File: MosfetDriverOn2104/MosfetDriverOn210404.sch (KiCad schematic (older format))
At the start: 88 parts, among them J1 I2C HDR, J10 ENCODER HDR, J11 CROSS CONN, J12 motor, J2 AVR-ISP-6, J3 I2C HDR, J4 Screw_Terminal_01x02, J5 I2C HDR, J6 UART HDR, J7 5V HDR, J8 GND HDR, J9 servo hdr, Q1 IRF540N, Q2 IRF540N, Q3 IRF540N, Q4 IRF540N, SW1 SW_Push, SW2 SW_DIP_x04, SW3 SW_Push, SW4 SW_Push, U1 LM2576HVS-ADJ, U2 L7805, U3 IR2104, U4 LM358, U5 IR2104, U6 ATmega328P-AU-MCU_Microchip_A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

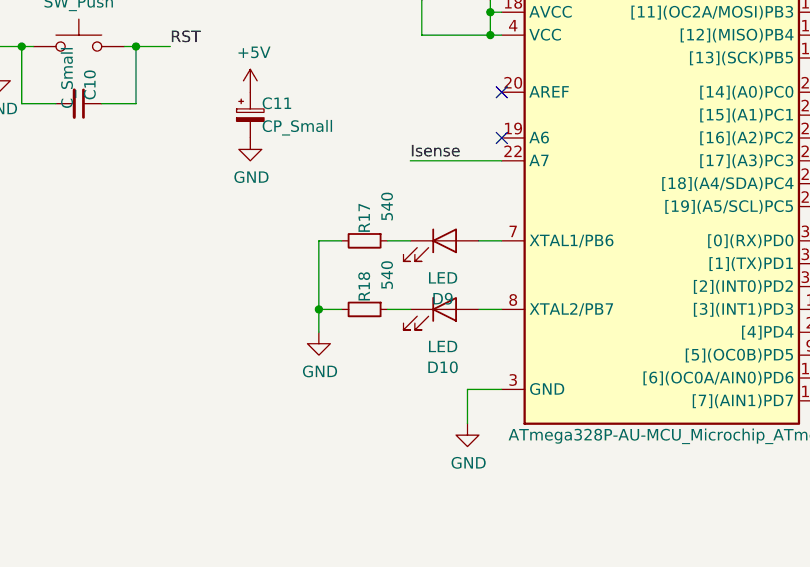
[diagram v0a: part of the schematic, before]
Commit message: yet to arrange!
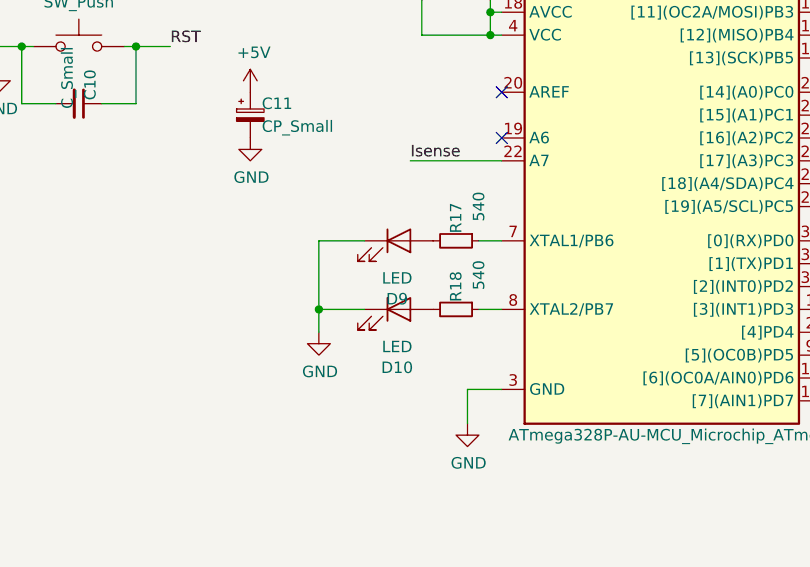
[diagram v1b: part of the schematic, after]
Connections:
- net GND: now also D10.1 (K), D9.1 (K); no longer R17.2, R18.2
- net at U6.7 (XTAL1/PB6): now also R17.1; no longer D9.2 (A)
- net at U6.8 (XTAL2/PB7): now also R18.1; no longer D10.2 (A)
- new net: D9.2 (A), R17.2
- new net: D10.2 (A), R18.2
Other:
- moved on the sheet: D10, D9, R17, R18
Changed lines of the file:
@@
 L Device:LED D?
 U 1 1 5BD9759E
-P 16800 850
+P 16600 850
 AR Path="/5BCF2976/5BD9759E" Ref="D?"  Part="1"
 AR Path="/5BD9759E" Ref="D9"  Part="1"
-F 0 "D9" H 16792 595 50  0000 C CNN
-F 1 "LED" H 16792 686 50  0000 C CNN
-F 2 "LED_SMD:LED_0805_2012Metric" H 16800 850 50  0001 C CNN
-F 3 "~" H 16800 850 50  0001 C CNN
-	1    16800 850
+F 0 "D9" H 16592 595 50  0000 C CNN
+F 1 "LED" H 16592 686 50  0000 C CNN
+F 2 "LED_SMD:LED_0805_2012Metric" H 16600 850 50  0001 C CNN
+F 3 "~" H 16600 850 50  0001 C CNN
+	1    16600 850
 	1    0    0    -1
 $EndComp
@@
 L Device:R_Small R?
 U 1 1 5BD975A5
-P 16450 850
+P 16850 850
 AR Path="/5BCF2976/5BD975A5" Ref="R?"  Part="1"
 AR Path="/5BD975A5" Ref="R17"  Part="1"
-F 0 "R17" H 16350 850 50  0000 C CNN
-F 1 "540" H 16300 950 50  0000 C CNN
-F 2 "Resistor_SMD:R_0805_2012Metric" H 16450 850 50  0001 C CNN
-F 3 "~" H 16450 850 50  0001 C CNN
-	1    16450 850
+F 0 "R17" H 16750 850 50  0000 C CNN
+F 1 "540" H 16700 950 50  0000 C CNN
+F 2 "Resistor_SMD:R_0805_2012Metric" H 16850 850 50  0001 C CNN
+F 3 "~" H 16850 850 50  0001 C CNN
+	1    16850 850
 	0    1    1    0
 $EndComp
@@
 L Device:LED D?
 U 1 1 5BD975B2
-P 16800 1150
+P 16600 1150
 AR Path="/5BCF2976/5BD975B2" Ref="D?"  Part="1"
 AR Path="/5BD975B2" Ref="D10"  Part="1"
-F 0 "D10" H 16792 895 50  0000 C CNN
-F 1 "LED" H 16792 986 50  0000 C CNN
-F 2 "LED_SMD:LED_0805_2012Metric" H 16800 1150 50  0001 C CNN
-F 3 "~" H 16800 1150 50  0001 C CNN
-	1    16800 1150
+F 0 "D10" H 16592 895 50  0000 C CNN
+F 1 "LED" H 16592 986 50  0000 C CNN
+F 2 "LED_SMD:LED_0805_2012Metric" H 16600 1150 50  0001 C CNN
+F 3 "~" H 16600 1150 50  0001 C CNN
+	1    16600 1150
 	1    0    0    -1
 $EndComp
@@
 L Device:R_Small R?
 U 1 1 5BD975B9
-P 16450 1150
+P 16850 1150
 AR Path="/5BCF2976/5BD975B9" Ref="R?"  Part="1"
 AR Path="/5BD975B9" Ref="R18"  Part="1"
-F 0 "R18" H 16350 1150 50  0000 C CNN
-F 1 "540" H 16300 1250 50  0000 C CNN
-F 2 "Resistor_SMD:R_0805_2012Metric" H 16450 1150 50  0001 C CNN
-F 3 "~" H 16450 1150 50  0001 C CNN
-	1    16450 1150
+F 0 "R18" H 16750 1150 50  0000 C CNN
+F 1 "540" H 16700 1250 50  0000 C CNN
+F 2 "Resistor_SMD:R_0805_2012Metric" H 16850 1150 50  0001 C CNN
+F 3 "~" H 16850 1150 50  0001 C CNN
+	1    16850 1150
 	0    1    1    0
 $EndComp
-Wire Wire Line
-	16650 1150 16550 1150
-Wire Wire Line
-	16650 850  16550 850
 Wire Wire Line
 	17050 850  16950 850
@@
 $EndComp
 Wire Wire Line
-	16350 850  16250 850
-Wire Wire Line
 	16250 850  16250 1150
-Wire Wire Line
-	16350 1150 16250 1150
 Connection ~ 16250 1150
 Wire Wire Line
@@
 	1    0    0    -1
 $EndComp
+Wire Wire Line
+	16250 850  16450 850
+Wire Wire Line
+	16250 1150 16450 1150
 $EndSCHEMATC

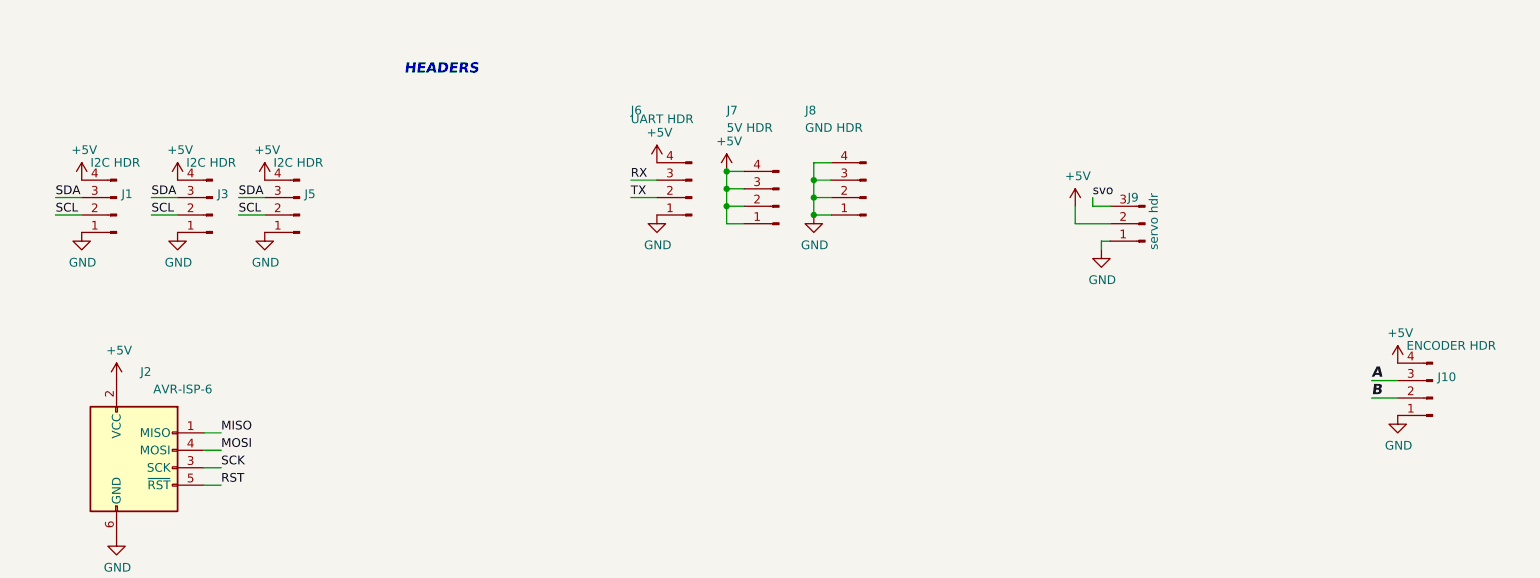
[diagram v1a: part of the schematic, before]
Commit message: necktie pattern
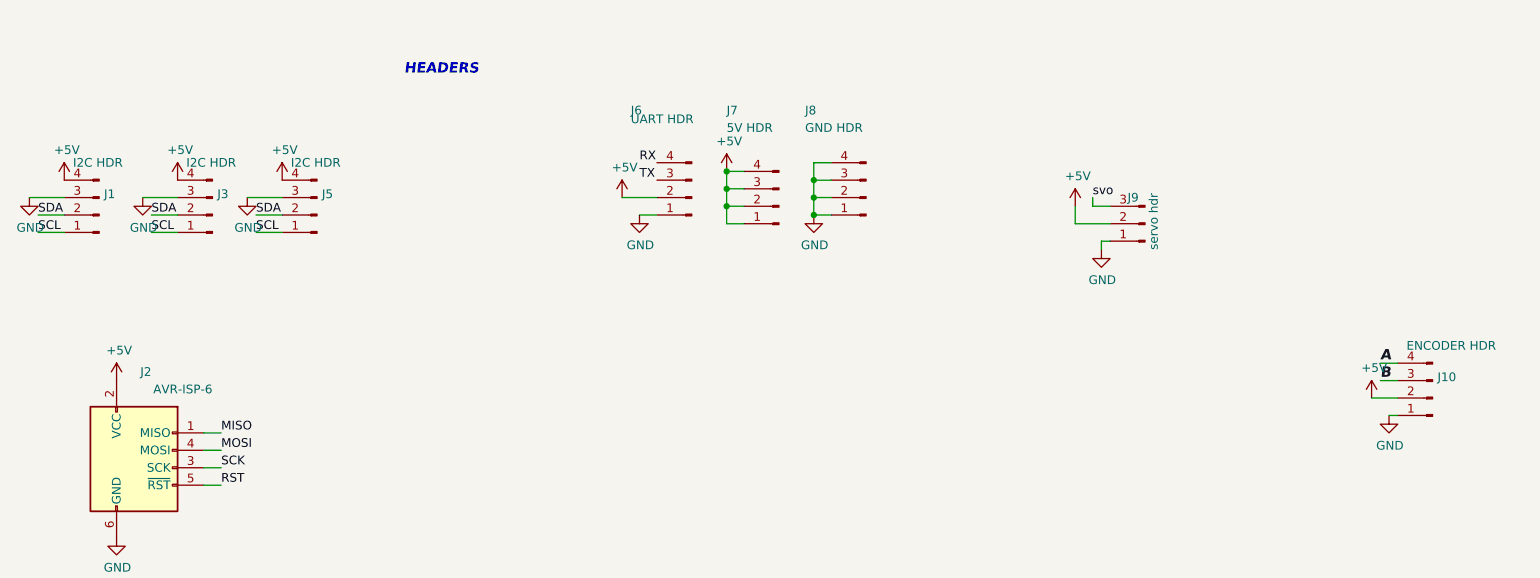
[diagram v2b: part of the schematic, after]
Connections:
- net +5V: now also J10.2 (Pin_2), J6.2 (Pin_2); no longer J10.4 (Pin_4), J6.4 (Pin_4)
- net A: now also J10.4 (Pin_4); no longer J10.3 (Pin_3)
- net B: now also J10.3 (Pin_3); no longer J10.2 (Pin_2)
- net GND: now also J1.3 (Pin_3), J3.3 (Pin_3), J5.3 (Pin_3); no longer J1.1 (Pin_1), J3.1 (Pin_1), J5.1 (Pin_1)
- net RX: no longer J6.3 (Pin_3)
- net SCL: now also J1.1 (Pin_1), J3.1 (Pin_1), J5.1 (Pin_1); no longer J1.2 (Pin_2), J3.2 (Pin_2), J5.2 (Pin_2)
- net SDA: now also J1.2 (Pin_2), J3.2 (Pin_2), J5.2 (Pin_2); no longer J1.3 (Pin_3), J3.3 (Pin_3), J5.3 (Pin_3)
- net TX: no longer J6.2 (Pin_2)
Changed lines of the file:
@@
 L power:+5V #PWR0118
 U 1 1 5BD95BFB
-P -5900 -550
+P -6100 -350
 AR Path="/5BD95BFB" Ref="#PWR0118"  Part="1"
 AR Path="/5BD0E604/5BD95BFB" Ref="#PWR?"  Part="1"
-F 0 "#PWR0118" H -5900 -700 50  0001 C CNN
-F 1 "+5V" H -5885 -377 50  0000 C CNN
-F 2 "" H -5900 -550 50  0001 C CNN
-F 3 "" H -5900 -550 50  0001 C CNN
-	1    -5900 -550
+F 0 "#PWR0118" H -6100 -500 50  0001 C CNN
+F 1 "+5V" H -6085 -177 50  0000 C CNN
+F 2 "" H -6100 -350 50  0001 C CNN
+F 3 "" H -6100 -350 50  0001 C CNN
+	1    -6100 -350
 	1    0    0    -1
 $EndComp
@@
 L power:GND #PWR0119
 U 1 1 5BD95C01
-P -5900 -250
+P -6000 -250
 AR Path="/5BD95C01" Ref="#PWR0119"  Part="1"
 AR Path="/5BD0E604/5BD95C01" Ref="#PWR?"  Part="1"
-F 0 "#PWR0119" H -5900 -500 50  0001 C CNN
-F 1 "GND" H -5895 -423 50  0000 C CNN
-F 2 "" H -5900 -250 50  0001 C CNN
-F 3 "" H -5900 -250 50  0001 C CNN
-	1    -5900 -250
-	1    0    0    -1
-$EndComp
-Text Label -6050 -450 0    50   ~ 0
+F 0 "#PWR0119" H -6000 -500 50  0001 C CNN
+F 1 "GND" H -5995 -423 50  0000 C CNN
+F 2 "" H -6000 -250 50  0001 C CNN
+F 3 "" H -6000 -250 50  0001 C CNN
+	1    -6000 -250
+	1    0    0    -1
+$EndComp
+Text Label -6000 -550 0    50   ~ 0
 RX
-Text Label -6050 -350 0    50   ~ 0
+Text Label -6000 -450 0    50   ~ 0
 TX
-Wire Wire Line
-	-6050 -450 -5900 -450
-Wire Wire Line
-	-5900 -350 -6050 -350
-$Comp
-L Connector:Conn_01x04_Male J5
-U 1 1 5BD95C0B
-P -7950 -250
-AR Path="/5BD95C0B" Ref="J5"  Part="1"
-AR Path="/5BD0E604/5BD95C0B" Ref="J?"  Part="1"
-F 0 "J5" H -7978 -370 50  0000 R CNN
-F 1 "I2C HDR" H -7800 -550 50  0000 R CNN
-F 2 "Connector_PinHeader_2.54mm:PinHeader_1x04_P2.54mm_Vertical" H -7950 -250 50  0001 C CNN
-F 3 "~" H -7950 -250 50  0001 C CNN
-	1    -7950 -250
-	-1   0    0    1
-$EndComp
-$Comp
-L power:+5V #PWR0120
-U 1 1 5BD95C12
-P -8150 -450
-AR Path="/5BD95C12" Ref="#PWR0120"  Part="1"
-AR Path="/5BD0E604/5BD95C12" Ref="#PWR?"  Part="1"
-F 0 "#PWR0120" H -8150 -600 50  0001 C CNN
-F 1 "+5V" H -8135 -277 50  0000 C CNN
-F 2 "" H -8150 -450 50  0001 C CNN
-F 3 "" H -8150 -450 50  0001 C CNN
-	1    -8150 -450
-	1    0    0    -1
-$EndComp
-$Comp
-L power:GND #PWR0121
-U 1 1 5BD95C18
-P -8150 -150
-AR Path="/5BD95C18" Ref="#PWR0121"  Part="1"
-AR Path="/5BD0E604/5BD95C18" Ref="#PWR?"  Part="1"
-F 0 "#PWR0121" H -8150 -400 50  0001 C CNN
-F 1 "GND" H -8145 -323 50  0000 C CNN
-F 2 "" H -8150 -150 50  0001 C CNN
-F 3 "" H -8150 -150 50  0001 C CNN
-	1    -8150 -150
-	1    0    0    -1
-$EndComp
-Text Label -8300 -350 0    50   ~ 0
-SDA
-Text Label -8300 -250 0    50   ~ 0
-SCL
-Wire Wire Line
-	-8150 -350 -8300 -350
-Wire Wire Line
-	-8300 -250 -8150 -250
 $Comp
 L Connector:Conn_01x04_Male J8
@@
 $EndComp
 $Comp
-L Connector:Conn_01x04_Male J1
-U 1 1 5BD95C64
-P -9000 -250
-AR Path="/5BD95C64" Ref="J1"  Part="1"
-AR Path="/5BD0E604/5BD95C64" Ref="J?"  Part="1"
-F 0 "J1" H -9028 -370 50  0000 R CNN
-F 1 "I2C HDR" H -8850 -550 50  0000 R CNN
-F 2 "Connector_PinHeader_2.54mm:PinHeader_1x04_P2.54mm_Vertical" H -9000 -250 50  0001 C CNN
-F 3 "~" H -9000 -250 50  0001 C CNN
-	1    -9000 -250
-	-1   0    0    1
-$EndComp
-$Comp
-L power:+5V #PWR0125
-U 1 1 5BD95C6B
-P -9200 -450
-AR Path="/5BD95C6B" Ref="#PWR0125"  Part="1"
-AR Path="/5BD0E604/5BD95C6B" Ref="#PWR?"  Part="1"
-F 0 "#PWR0125" H -9200 -600 50  0001 C CNN
-F 1 "+5V" H -9185 -277 50  0000 C CNN
-F 2 "" H -9200 -450 50  0001 C CNN
-F 3 "" H -9200 -450 50  0001 C CNN
-	1    -9200 -450
-	1    0    0    -1
-$EndComp
-$Comp
-L power:GND #PWR0126
-U 1 1 5BD95C71
-P -9200 -150
-AR Path="/5BD95C71" Ref="#PWR0126"  Part="1"
-AR Path="/5BD0E604/5BD95C71" Ref="#PWR?"  Part="1"
-F 0 "#PWR0126" H -9200 -400 50  0001 C CNN
-F 1 "GND" H -9195 -323 50  0000 C CNN
-F 2 "" H -9200 -150 50  0001 C CNN
-F 3 "" H -9200 -150 50  0001 C CNN
-	1    -9200 -150
-	1    0    0    -1
-$EndComp
-Text Label -9350 -350 0    50   ~ 0
-SDA
-Text Label -9350 -250 0    50   ~ 0
-SCL
-Wire Wire Line
-	-9200 -350 -9350 -350
-Wire Wire Line
-	-9350 -250 -9200 -250
-$Comp
 L Connector:Conn_01x04_Male J3
 U 1 1 5BD95C7B
@@
 L power:GND #PWR0128
 U 1 1 5BD95C88
-P -8650 -150
+P -8850 -350
 AR Path="/5BD95C88" Ref="#PWR0128"  Part="1"
 AR Path="/5BD0E604/5BD95C88" Ref="#PWR?"  Part="1"
-F 0 "#PWR0128" H -8650 -400 50  0001 C CNN
-F 1 "GND" H -8645 -323 50  0000 C CNN
-F 2 "" H -8650 -150 50  0001 C CNN
-F 3 "" H -8650 -150 50  0001 C CNN
-	1    -8650 -150
-	1    0    0    -1
-$EndComp
-Text Label -8800 -350 0    50   ~ 0
+F 0 "#PWR0128" H -8850 -600 50  0001 C CNN
+F 1 "GND" H -8845 -523 50  0000 C CNN
+F 2 "" H -8850 -350 50  0001 C CNN
+F 3 "" H -8850 -350 50  0001 C CNN
+	1    -8850 -350
+	1    0    0    -1
+$EndComp
+Text Label -8800 -250 0    50   ~ 0
 SDA
-Text Label -8800 -250 0    50   ~ 0
+Text Label -8800 -150 0    50   ~ 0
 SCL
-Wire Wire Line
-	-8650 -350 -8800 -350
 Wire Wire Line
 	-8800 -250 -8650 -250
@@
 L power:+5V #PWR0129
 U 1 1 5BD95C9C
-P -1650 600
+P -1800 800
 AR Path="/5BD95C9C" Ref="#PWR0129"  Part="1"
 AR Path="/5BD0E604/5BD95C9C" Ref="#PWR?"  Part="1"
-F 0 "#PWR0129" H -1650 450 50  0001 C CNN
-F 1 "+5V" H -1635 773 50  0000 C CNN
-F 2 "" H -1650 600 50  0001 C CNN
-F 3 "" H -1650 600 50  0001 C CNN
-	1    -1650 600
+F 0 "#PWR0129" H -1800 650 50  0001 C CNN
+F 1 "+5V" H -1785 973 50  0000 C CNN
+F 2 "" H -1800 800 50  0001 C CNN
+F 3 "" H -1800 800 50  0001 C CNN
+	1    -1800 800
 	1    0    0    -1
 $EndComp
@@
 L power:GND #PWR0130
 U 1 1 5BD95CA2
-P -1650 900
+P -1700 900
 AR Path="/5BD95CA2" Ref="#PWR0130"  Part="1"
 AR Path="/5BD0E604/5BD95CA2" Ref="#PWR?"  Part="1"
-F 0 "#PWR0130" H -1650 650 50  0001 C CNN
-F 1 "GND" H -1645 727 50  0000 C CNN
-F 2 "" H -1650 900 50  0001 C CNN
-F 3 "" H -1650 900 50  0001 C CNN
-	1    -1650 900
-	1    0    0    -1
-$EndComp
-Wire Wire Line
-	-1650 700  -1800 700
+F 0 "#PWR0130" H -1700 650 50  0001 C CNN
+F 1 "GND" H -1695 727 50  0000 C CNN
+F 2 "" H -1700 900 50  0001 C CNN
+F 3 "" H -1700 900 50  0001 C CNN
+	1    -1700 900
+	1    0    0    -1
+$EndComp
 Wire Wire Line
 	-1800 800  -1650 800
-Text Label -1800 700  0    59   Italic 12
+Text Label -1750 600  0    59   Italic 12
 A
-Text Label -1800 800  0    59   Italic 12
+Text Label -1750 700  0    59   Italic 12
 B
 $Comp
@@
 Wire Wire Line
 	16250 1150 16450 1150
+Wire Wire Line
+	-6100 -350 -5900 -350
+Wire Wire Line
+	-5900 -250 -6000 -250
+Wire Wire Line
+	-1750 600  -1650 600
+Wire Wire Line
+	-1750 700  -1650 700
+Wire Wire Line
+	-1650 900  -1700 900
+Wire Wire Line
+	-8800 -150 -8650 -150
+Wire Wire Line
+	-8850 -350 -8650 -350
+$Comp
+L Connector:Conn_01x04_Male J5
+U 1 1 5BFA199C
+P -7850 -250
+AR Path="/5BFA199C" Ref="J5"  Part="1"
+AR Path="/5BD0E604/5BFA199C" Ref="J?"  Part="1"
+F 0 "J5" H -7878 -370 50  0000 R CNN
+F 1 "I2C HDR" H -7700 -550 50  0000 R CNN
+F 2 "Connector_PinHeader_2.54mm:PinHeader_1x04_P2.54mm_Vertical" H -7850 -250 50  0001 C CNN
+F 3 "~" H -7850 -250 50  0001 C CNN
+	1    -7850 -250
+	-1   0    0    1
+$EndComp
+$Comp
+L power:+5V #PWR0120
+U 1 1 5BFA19A3
+P -8050 -450
+AR Path="/5BFA19A3" Ref="#PWR0120"  Part="1"
+AR Path="/5BD0E604/5BFA19A3" Ref="#PWR?"  Part="1"
+F 0 "#PWR0120" H -8050 -600 50  0001 C CNN
+F 1 "+5V" H -8035 -277 50  0000 C CNN
+F 2 "" H -8050 -450 50  0001 C CNN
+F 3 "" H -8050 -450 50  0001 C CNN
+	1    -8050 -450
+	1    0    0    -1
+$EndComp
+$Comp
+L power:GND #PWR0121
+U 1 1 5BFA19A9
+P -8250 -350
+AR Path="/5BFA19A9" Ref="#PWR0121"  Part="1"
+AR Path="/5BD0E604/5BFA19A9" Ref="#PWR?"  Part="1"
+F 0 "#PWR0121" H -8250 -600 50  0001 C CNN
+F 1 "GND" H -8245 -523 50  0000 C CNN
+F 2 "" H -8250 -350 50  0001 C CNN
+F 3 "" H -8250 -350 50  0001 C CNN
+	1    -8250 -350
+	1    0    0    -1
+$EndComp
+Text Label -8200 -250 0    50   ~ 0
+SDA
+Text Label -8200 -150 0    50   ~ 0
+SCL
+Wire Wire Line
+	-8200 -250 -8050 -250
+Wire Wire Line
+	-8200 -150 -8050 -150
+Wire Wire Line
+	-8250 -350 -8050 -350
+$Comp
+L Connector:Conn_01x04_Male J1
+U 1 1 5BFB80C0
+P -9100 -250
+AR Path="/5BFB80C0" Ref="J1"  Part="1"
+AR Path="/5BD0E604/5BFB80C0" Ref="J?"  Part="1"
+F 0 "J1" H -9128 -370 50  0000 R CNN
+F 1 "I2C HDR" H -8950 -550 50  0000 R CNN
+F 2 "Connector_PinHeader_2.54mm:PinHeader_1x04_P2.54mm_Vertical" H -9100 -250 50  0001 C CNN
+F 3 "~" H -9100 -250 50  0001 C CNN
+	1    -9100 -250
+	-1   0    0    1
+$EndComp
+$Comp
+L power:+5V #PWR0125
+U 1 1 5BFB80C7
+P -9300 -450
+AR Path="/5BFB80C7" Ref="#PWR0125"  Part="1"
+AR Path="/5BD0E604/5BFB80C7" Ref="#PWR?"  Part="1"
+F 0 "#PWR0125" H -9300 -600 50  0001 C CNN
+F 1 "+5V" H -9285 -277 50  0000 C CNN
+F 2 "" H -9300 -450 50  0001 C CNN
+F 3 "" H -9300 -450 50  0001 C CNN
+	1    -9300 -450
+	1    0    0    -1
+$EndComp
+$Comp
+L power:GND #PWR0126
+U 1 1 5BFB80CD
+P -9500 -350
+AR Path="/5BFB80CD" Ref="#PWR0126"  Part="1"
+AR Path="/5BD0E604/5BFB80CD" Ref="#PWR?"  Part="1"
+F 0 "#PWR0126" H -9500 -600 50  0001 C CNN
+F 1 "GND" H -9495 -523 50  0000 C CNN
+F 2 "" H -9500 -350 50  0001 C CNN
+F 3 "" H -9500 -350 50  0001 C CNN
+	1    -9500 -350
+	1    0    0    -1
+$EndComp
+Text Label -9450 -250 0    50   ~ 0
+SDA
+Text Label -9450 -150 0    50   ~ 0
+SCL
+Wire Wire Line
+	-9450 -250 -9300 -250
+Wire Wire Line
+	-9450 -150 -9300 -150
+Wire Wire Line
+	-9500 -350 -9300 -350
 $EndSCHEMATC
